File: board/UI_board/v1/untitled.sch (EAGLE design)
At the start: 19 parts

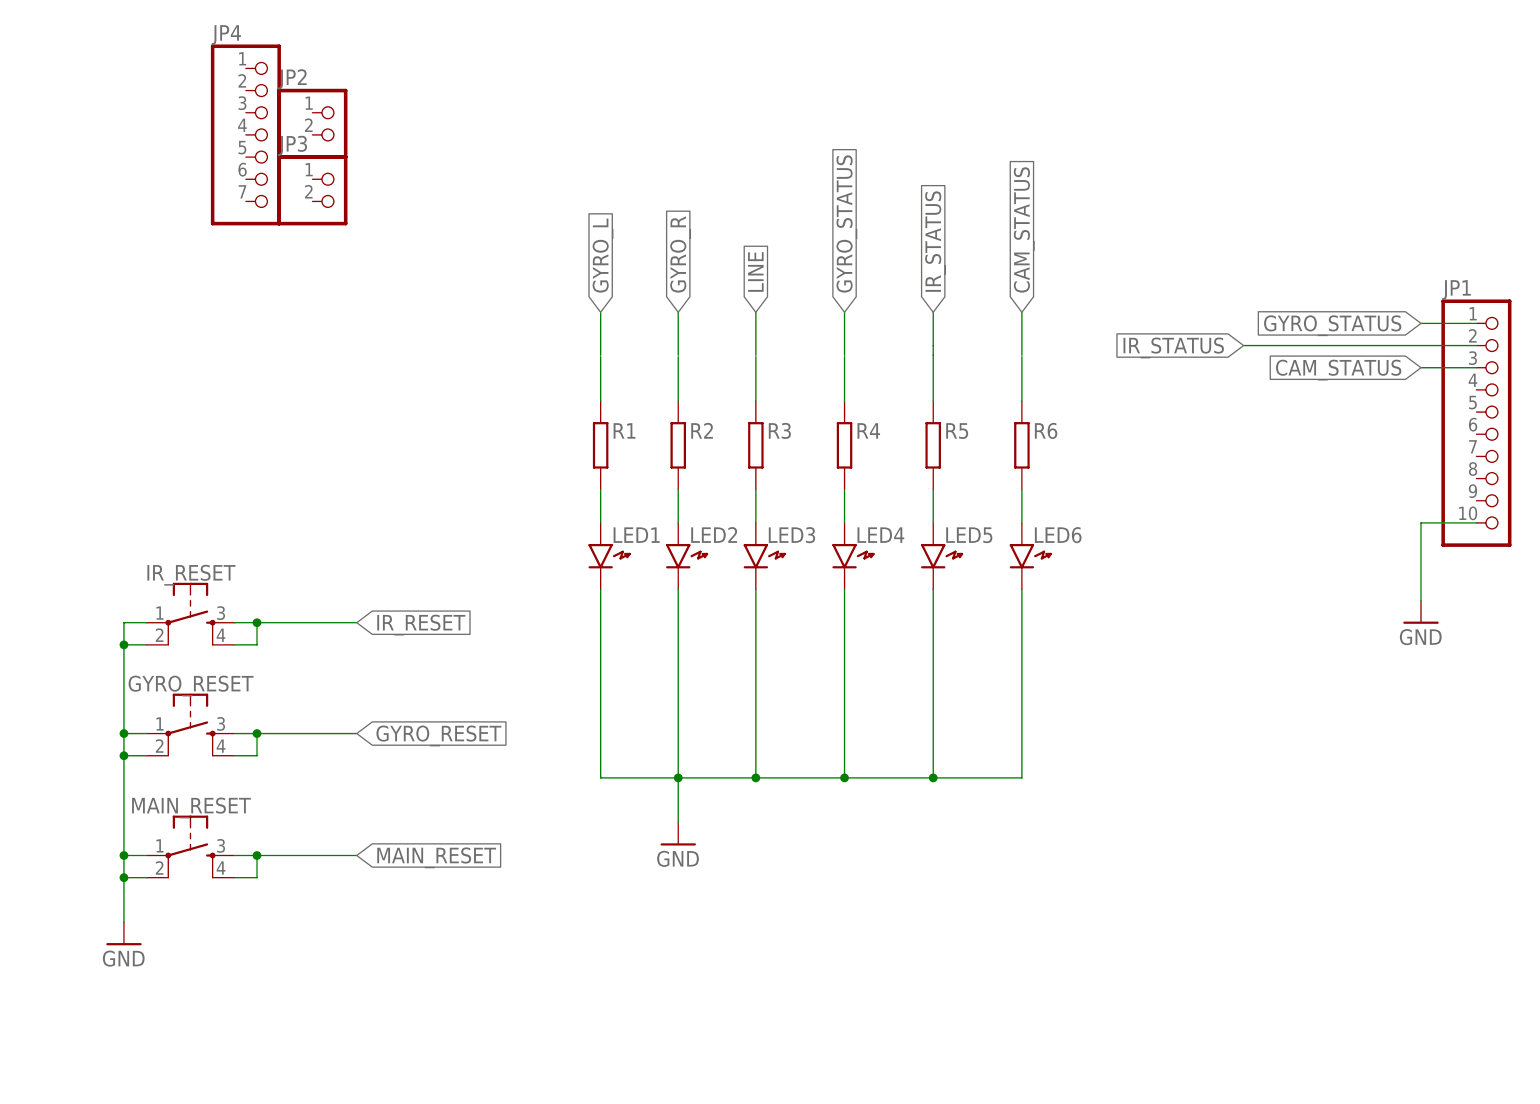
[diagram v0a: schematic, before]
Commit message: complete wiring
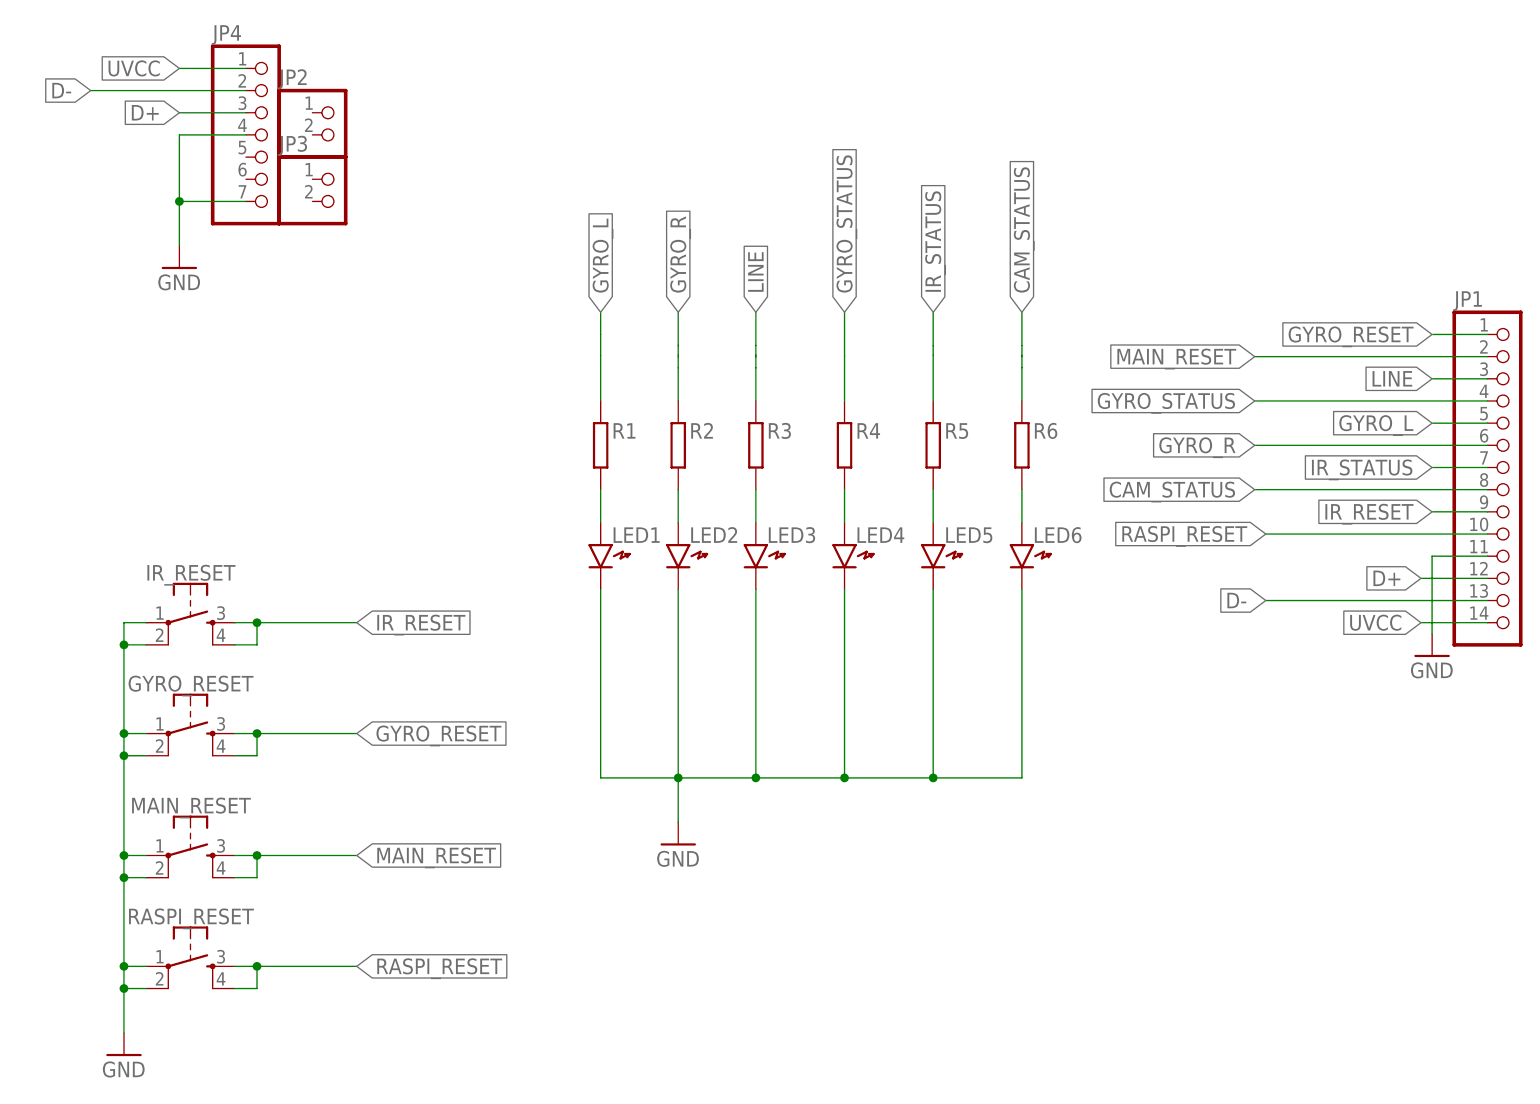
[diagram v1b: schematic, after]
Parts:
- added RASPI_RESET: (no value), SparkFun-Switches:MOMENTARY-SWITCH-SPST-2-SMD-5.2MM
- JP1: device pinhead:PINHD-1X10 -> pinhead:PINHD-1X14
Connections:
- removed net N$10: R2.1
- removed net N$11: R1.1
- removed net N$7: R6.1
- removed net N$8: R4.1
- removed net N$9: R3.1
- new net D+: JP1.12, JP4.3
- new net D-: JP1.13, JP4.2
- new net GYRO_L: JP1.5, R1.1
- new net GYRO_R: JP1.6, R2.1
- new net LINE: JP1.3, R3.1
- new net RASPI_RESET: JP1.10, RASPI_RESET.3, RASPI_RESET.4
- new net UVCC: JP1.14, JP4.1
- net CAM_STATUS: now also JP1.8, R6.1; no longer JP1.3
- net GND: now also JP1.11, JP4.4, JP4.7, RASPI_RESET.1, RASPI_RESET.2; no longer JP1.10
- net GYRO_RESET: now also JP1.1
- net GYRO_STATUS: now also JP1.4, R4.1; no longer JP1.1
- net IR_RESET: now also JP1.9
- net IR_STATUS: now also JP1.7; no longer JP1.2
- net MAIN_RESET: now also JP1.2
